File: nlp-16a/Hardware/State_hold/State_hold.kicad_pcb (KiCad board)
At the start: 2 copper layers, 45.7 x 99.1 mm, 63 parts, among them J1 Conn_01x08_Male, J2 Conn_01x08_Male, J3 Conn_01x08_Male, J4 Conn_01x08_Male, J5 Conn_01x08_Male, J6 Conn_01x08_Male, J7 Conn_01x08_Male, J8 Conn_01x08_Male, J9 Conn_01x02_Male, U1 CD74HC00, U10 CD74HC00, U11 CD74HC00, U12 CD74HC00, U2 CD74HC00, U3 CD74HC00, U4 CD74HC00, U5 CD74HC00, U6 CD74HC00, U7 CD74HC00, U8 CD74HC00, U9 CD74HC00

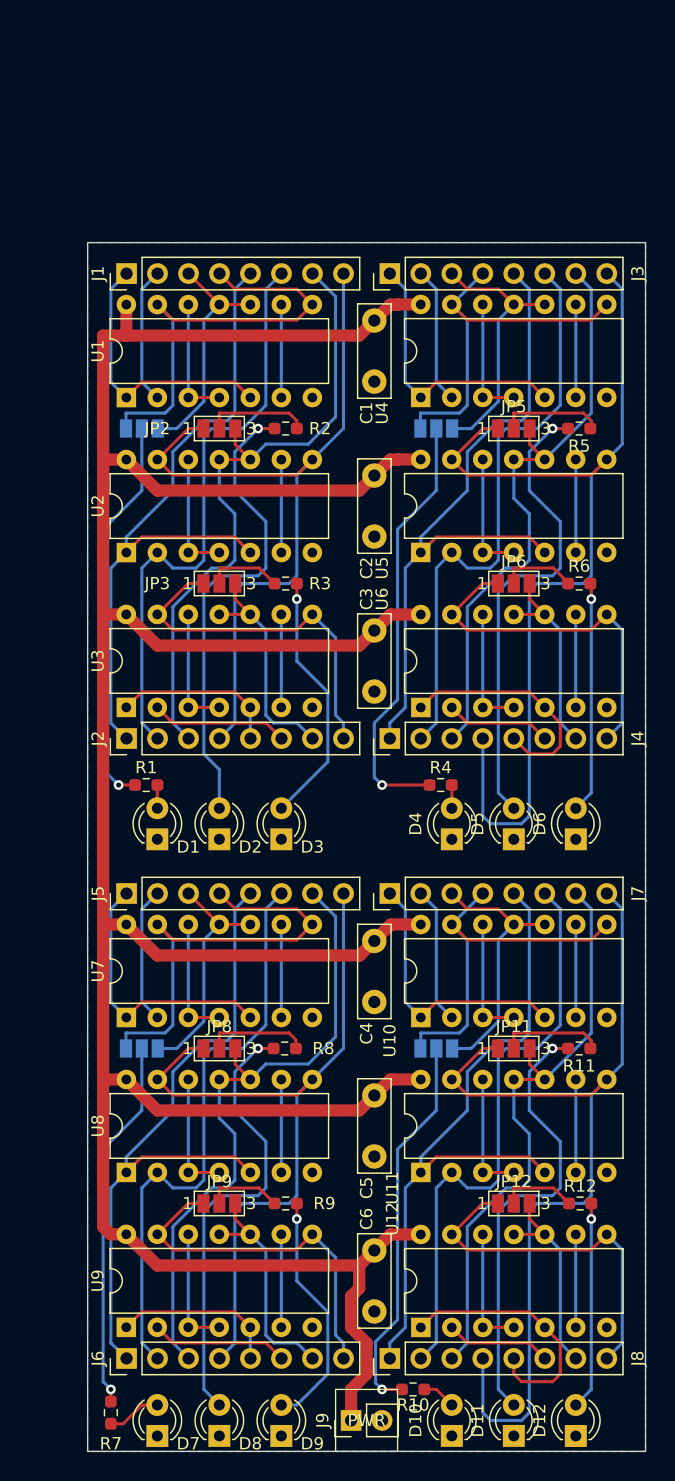
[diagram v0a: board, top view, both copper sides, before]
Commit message: ステート保持ラッチ再設計．おそらく問題無し
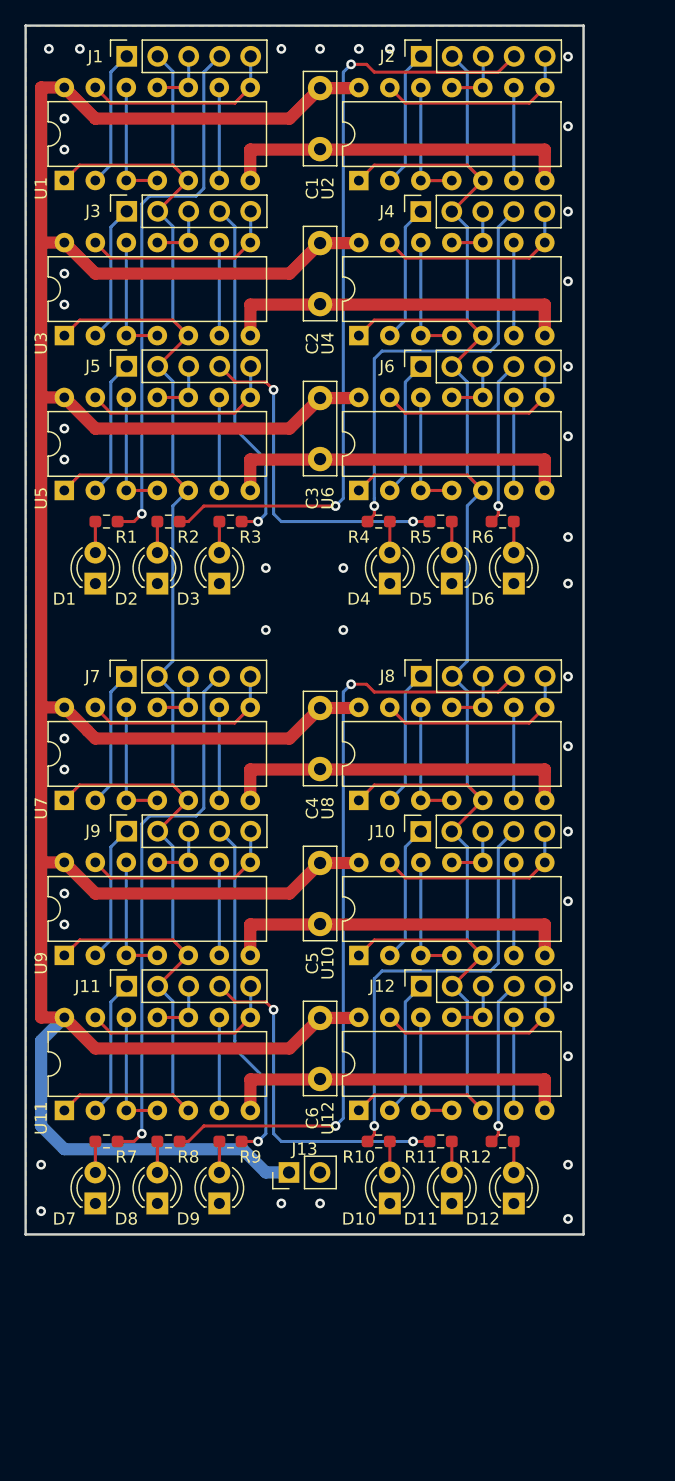
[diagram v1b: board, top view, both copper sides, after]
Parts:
- removed JP1, JP10, JP11, JP12, JP2, JP3, JP4, JP5, JP6, JP7, JP8, JP9: Jumper_3_Open, Jumper:SolderJumper-3_P1.3mm_Open_Pad1.0x1.5mm_NumberLabels
- added J10: Conn_01x05_Female, Connector_PinSocket_2.54mm:PinSocket_1x05_P2.54mm_Vertical, F.Cu at (229.9, 107.3)
- added J11: Conn_01x05_Female, Connector_PinSocket_2.54mm:PinSocket_1x05_P2.54mm_Vertical, F.Cu at (205.8, 120.0)
- added J12: Conn_01x05_Female, Connector_PinSocket_2.54mm:PinSocket_1x05_P2.54mm_Vertical, F.Cu at (229.9, 120.0)
- added J13: Conn_01x02_Male, Connector_PinHeader_2.54mm:PinHeader_1x02_P2.54mm_Vertical, F.Cu at (219.1, 135.3)
- J1, J2, J3, J4, J5, J6, J7, J8: value Conn_01x08_Male -> Conn_01x05_Female; footprint Connector_PinHeader_2.54mm:PinHeader_1x08_P2.54mm_Vertical -> Connector_PinSocket_2.54mm:PinSocket_1x05_P2.54mm_Vertical
- J9: value Conn_01x02_Male -> Conn_01x05_Female; footprint Connector_PinHeader_2.54mm:PinHeader_1x02_P2.54mm_Vertical -> Connector_PinSocket_2.54mm:PinSocket_1x05_P2.54mm_Vertical
- moved J6 84.8 mm to (229.9, 69.2)
- moved J2 60.9 mm to (229.9, 43.8)
- moved J8 56.0 mm to (229.9, 94.6)
- moved J9 51.7 mm to (205.8, 107.3)
- moved J4 43.3 mm to (229.9, 56.5)
- moved J5 43.2 mm to (205.8, 69.2)
- moved U8 35.9 mm to (224.8, 104.8)
- moved U2 35.9 mm to (224.8, 54.0)
- moved U9 30.9 mm to (200.7, 117.5)
- moved U3 30.9 mm to (200.7, 66.7)
- moved U11 29.6 mm to (200.7, 130.2)
- moved U5 29.6 mm to (200.7, 79.4)
- moved J7 28.0 mm to (205.7, 94.6)
- moved R7 22.2 mm to (204.1, 132.7), turned to 180 degrees
- moved R4 22.2 mm to (226.4, 81.9)
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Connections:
- net /State_hold_unit0/Q renamed /State_latch0/Q
- J1 pad 1: /State_hold_unit0/Gate -> /State_latch0/D
- J1 pad 2: /State_hold_unit0/D -> /State_latch0/Gate
- J1 pad 4: /State_hold_unit0/~{Q} -> /State_latch0/LED
- J1 pad 5: /State_hold_unit1/Gate -> /State_latch0/~{Q}
- J2 pad 1: /State_hold_unit1/Gate -> /State_latch1/D
- J2 pad 2: /State_hold_unit1/D -> /State_latch1/Gate
- J2 pad 3: /State_hold_unit1/Q -> /State_latch1/Q
- J2 pad 4: /State_hold_unit1/~{Q} -> /State_latch1/LED
- J2 pad 5: /State_hold_unit2/Gate -> /State_latch1/~{Q}
- J3 pad 1: /State_hold_unit3/Gate -> /State_latch2/D
- J3 pad 2: /State_hold_unit3/D -> /State_latch0/Gate
- J3 pad 3: /State_hold_unit3/Q -> /State_latch2/Q
- J3 pad 4: /State_hold_unit3/~{Q} -> /State_latch2/LED
- J3 pad 5: /State_hold_unit4/Gate -> /State_latch2/~{Q}
- J4 pad 1: /State_hold_unit4/Gate -> /State_latch3/D
- J4 pad 2: /State_hold_unit4/D -> /State_latch1/Gate
- J4 pad 3: /State_hold_unit4/Q -> /State_latch3/Q
- J4 pad 4: /State_hold_unit4/~{Q} -> /State_latch3/LED
- J4 pad 5: /State_hold_unit5/Gate -> /State_latch3/~{Q}
- J5 pad 1: /State_hold_unit6/Gate -> /State_latch4/D
- J5 pad 2: /State_hold_unit6/D -> /State_latch0/Gate
- J5 pad 3: /State_hold_unit6/Q -> /State_latch4/Q
- J5 pad 4: /State_hold_unit6/~{Q} -> /State_latch4/LED
- J5 pad 5: /State_hold_unit7/Gate -> /State_latch4/~{Q}
- J6 pad 1: /State_hold_unit7/Gate -> /State_latch5/D
- J6 pad 2: /State_hold_unit7/D -> /State_latch1/Gate
- J6 pad 3: /State_hold_unit7/Q -> /State_latch5/Q
- J6 pad 4: /State_hold_unit7/~{Q} -> /State_latch5/LED
- J6 pad 5: /State_hold_unit8/Gate -> /State_latch5/~{Q}
- J7 pad 1: /State_hold_unit9/Gate -> /State_latch6/D
- J7 pad 2: /State_hold_unit9/D -> /State_latch0/Gate
- J7 pad 3: /State_hold_unit9/Q -> /State_latch6/Q
- J7 pad 4: /State_hold_unit9/~{Q} -> /State_latch6/LED
- J7 pad 5: /State_hold_unit10/Gate -> /State_latch6/~{Q}
- J8 pad 1: /State_hold_unit10/Gate -> /State_latch7/D
- J8 pad 2: /State_hold_unit10/D -> /State_latch1/Gate
- J8 pad 3: /State_hold_unit10/Q -> /State_latch7/Q
- J8 pad 4: /State_hold_unit10/~{Q} -> /State_latch7/LED
- J8 pad 5: /State_hold_unit11/Gate -> /State_latch7/~{Q}
- J9 pad 1: VCC -> /State_latch8/D
- J9 pad 2: GND -> /State_latch0/Gate
- R1 pad 1: Net-(JP1-Pad2) -> /State_latch0/LED
- R10 pad 1: Net-(JP10-Pad2) -> /State_latch9/LED
- R11 pad 1: Net-(JP11-Pad2) -> /State_latch10/LED
- R12 pad 1: Net-(JP12-Pad2) -> /State_latch11/LED
- R2 pad 1: Net-(JP2-Pad2) -> /State_latch1/LED
- R3 pad 1: Net-(JP3-Pad2) -> /State_latch2/LED
- R4 pad 1: Net-(JP4-Pad2) -> /State_latch3/LED
- R5 pad 1: Net-(JP5-Pad2) -> /State_latch4/LED
- R6 pad 1: Net-(JP6-Pad2) -> /State_latch5/LED
- R7 pad 1: Net-(JP7-Pad2) -> /State_latch6/LED
- R8 pad 1: Net-(JP8-Pad2) -> /State_latch7/LED
- R9 pad 1: Net-(JP9-Pad2) -> /State_latch8/LED
- U1 pad 1: /State_hold_unit0/Gate -> /State_latch0/Gate
- U1 pad 13: /State_hold_unit0/~{Q} -> /State_latch0/~{Q}
- U1 pad 2: /State_hold_unit0/D -> /State_latch0/D
- U1 pad 5: /State_hold_unit0/Gate -> /State_latch0/Gate
- U1 pad 8: /State_hold_unit0/~{Q} -> /State_latch0/~{Q}
- U10 pad 1: /State_hold_unit9/Gate -> /State_latch1/Gate
- U10 pad 10: /State_hold_unit9/Q -> /State_latch9/Q
- U10 pad 11: /State_hold_unit9/Q -> /State_latch9/Q
- U10 pad 13: /State_hold_unit9/~{Q} -> /State_latch9/~{Q}
- U10 pad 2: /State_hold_unit9/D -> /State_latch9/D
- U10 pad 5: /State_hold_unit9/Gate -> /State_latch1/Gate
- U10 pad 8: /State_hold_unit9/~{Q} -> /State_latch9/~{Q}
- U11 pad 1: /State_hold_unit10/Gate -> /State_latch0/Gate
- U11 pad 10: /State_hold_unit10/Q -> /State_latch10/Q
- U11 pad 11: /State_hold_unit10/Q -> /State_latch10/Q
- U11 pad 13: /State_hold_unit10/~{Q} -> /State_latch10/~{Q}
- U11 pad 2: /State_hold_unit10/D -> /State_latch10/D
- U11 pad 5: /State_hold_unit10/Gate -> /State_latch0/Gate
- U11 pad 8: /State_hold_unit10/~{Q} -> /State_latch10/~{Q}
- U12 pad 1: /State_hold_unit11/Gate -> /State_latch1/Gate
- U12 pad 10: /State_hold_unit11/Q -> /State_latch11/Q
- U12 pad 11: /State_hold_unit11/Q -> /State_latch11/Q
- U12 pad 13: /State_hold_unit11/~{Q} -> /State_latch11/~{Q}
- U12 pad 2: /State_hold_unit11/D -> /State_latch11/D
- U12 pad 5: /State_hold_unit11/Gate -> /State_latch1/Gate
- U12 pad 8: /State_hold_unit11/~{Q} -> /State_latch11/~{Q}
- U2 pad 1: /State_hold_unit1/Gate -> /State_latch1/Gate
- U2 pad 10: /State_hold_unit1/Q -> /State_latch1/Q
- U2 pad 11: /State_hold_unit1/Q -> /State_latch1/Q
- U2 pad 13: /State_hold_unit1/~{Q} -> /State_latch1/~{Q}
- U2 pad 2: /State_hold_unit1/D -> /State_latch1/D
- U2 pad 5: /State_hold_unit1/Gate -> /State_latch1/Gate
- U2 pad 8: /State_hold_unit1/~{Q} -> /State_latch1/~{Q}
- U3 pad 1: /State_hold_unit2/Gate -> /State_latch0/Gate
- U3 pad 10: /State_hold_unit2/Q -> /State_latch2/Q
- U3 pad 11: /State_hold_unit2/Q -> /State_latch2/Q
- U3 pad 13: /State_hold_unit2/~{Q} -> /State_latch2/~{Q}
- U3 pad 2: /State_hold_unit2/D -> /State_latch2/D
- U3 pad 5: /State_hold_unit2/Gate -> /State_latch0/Gate
- U3 pad 8: /State_hold_unit2/~{Q} -> /State_latch2/~{Q}
- U4 pad 1: /State_hold_unit3/Gate -> /State_latch1/Gate
- U4 pad 10: /State_hold_unit3/Q -> /State_latch3/Q
- U4 pad 11: /State_hold_unit3/Q -> /State_latch3/Q
- U4 pad 13: /State_hold_unit3/~{Q} -> /State_latch3/~{Q}
- U4 pad 2: /State_hold_unit3/D -> /State_latch3/D
- U4 pad 5: /State_hold_unit3/Gate -> /State_latch1/Gate
- U4 pad 8: /State_hold_unit3/~{Q} -> /State_latch3/~{Q}
- U5 pad 1: /State_hold_unit4/Gate -> /State_latch0/Gate
- U5 pad 10: /State_hold_unit4/Q -> /State_latch4/Q
- U5 pad 11: /State_hold_unit4/Q -> /State_latch4/Q
- U5 pad 13: /State_hold_unit4/~{Q} -> /State_latch4/~{Q}
- U5 pad 2: /State_hold_unit4/D -> /State_latch4/D
- U5 pad 5: /State_hold_unit4/Gate -> /State_latch0/Gate
- U5 pad 8: /State_hold_unit4/~{Q} -> /State_latch4/~{Q}
- U6 pad 1: /State_hold_unit5/Gate -> /State_latch1/Gate
- U6 pad 10: /State_hold_unit5/Q -> /State_latch5/Q
- U6 pad 11: /State_hold_unit5/Q -> /State_latch5/Q
- U6 pad 13: /State_hold_unit5/~{Q} -> /State_latch5/~{Q}
- U6 pad 2: /State_hold_unit5/D -> /State_latch5/D
- U6 pad 5: /State_hold_unit5/Gate -> /State_latch1/Gate
- U6 pad 8: /State_hold_unit5/~{Q} -> /State_latch5/~{Q}
- U7 pad 1: /State_hold_unit6/Gate -> /State_latch0/Gate
- U7 pad 10: /State_hold_unit6/Q -> /State_latch6/Q
- U7 pad 11: /State_hold_unit6/Q -> /State_latch6/Q
- U7 pad 13: /State_hold_unit6/~{Q} -> /State_latch6/~{Q}
- U7 pad 2: /State_hold_unit6/D -> /State_latch6/D
- U7 pad 5: /State_hold_unit6/Gate -> /State_latch0/Gate
- U7 pad 8: /State_hold_unit6/~{Q} -> /State_latch6/~{Q}
- U8 pad 1: /State_hold_unit7/Gate -> /State_latch1/Gate
- U8 pad 10: /State_hold_unit7/Q -> /State_latch7/Q
- U8 pad 11: /State_hold_unit7/Q -> /State_latch7/Q
- U8 pad 13: /State_hold_unit7/~{Q} -> /State_latch7/~{Q}
- U8 pad 2: /State_hold_unit7/D -> /State_latch7/D
- U8 pad 5: /State_hold_unit7/Gate -> /State_latch1/Gate
- U8 pad 8: /State_hold_unit7/~{Q} -> /State_latch7/~{Q}
- U9 pad 1: /State_hold_unit8/Gate -> /State_latch0/Gate
- U9 pad 10: /State_hold_unit8/Q -> /State_latch8/Q
- U9 pad 11: /State_hold_unit8/Q -> /State_latch8/Q
- U9 pad 13: /State_hold_unit8/~{Q} -> /State_latch8/~{Q}
- U9 pad 2: /State_hold_unit8/D -> /State_latch8/D
- U9 pad 5: /State_hold_unit8/Gate -> /State_latch0/Gate
- U9 pad 8: /State_hold_unit8/~{Q} -> /State_latch8/~{Q}
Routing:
- net GND: track 0.00 -> 175.2 mm, vias 0 -> 40
- net /State_latch1/Gate: track 0.00 -> 165.1 mm
- net /State_latch0/Gate: track 0.00 -> 165.1 mm
- net /State_hold_unit4/~{Q}: track 79.6 -> 0.00 mm
- net /State_hold_unit10/~{Q}: track 75.8 -> 0.00 mm
- net /State_latch7/LED: track 0.00 -> 64.2 mm, vias 0 -> 2
- net /State_latch1/LED: track 0.00 -> 64.2 mm, vias 0 -> 2
- net /State_hold_unit7/~{Q}: track 63.1 -> 0.00 mm
- net /State_hold_unit1/~{Q}: track 63.1 -> 0.00 mm
- net /State_hold_unit7/Gate: track 55.7 -> 0.00 mm
- net /State_hold_unit1/Gate: track 55.7 -> 0.00 mm
- net /State_hold_unit4/Gate: track 55.7 -> 0.00 mm
- net /State_hold_unit10/Gate: track 55.7 -> 0.00 mm
- net /State_hold_unit7/Q: track 53.3 -> 0.00 mm
- net /State_hold_unit1/Q: track 53.3 -> 0.00 mm
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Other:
- board text removed: "PWR"
